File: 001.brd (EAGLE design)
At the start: 100 x 80 mm, 16 parts, among them IC1 74HC148N

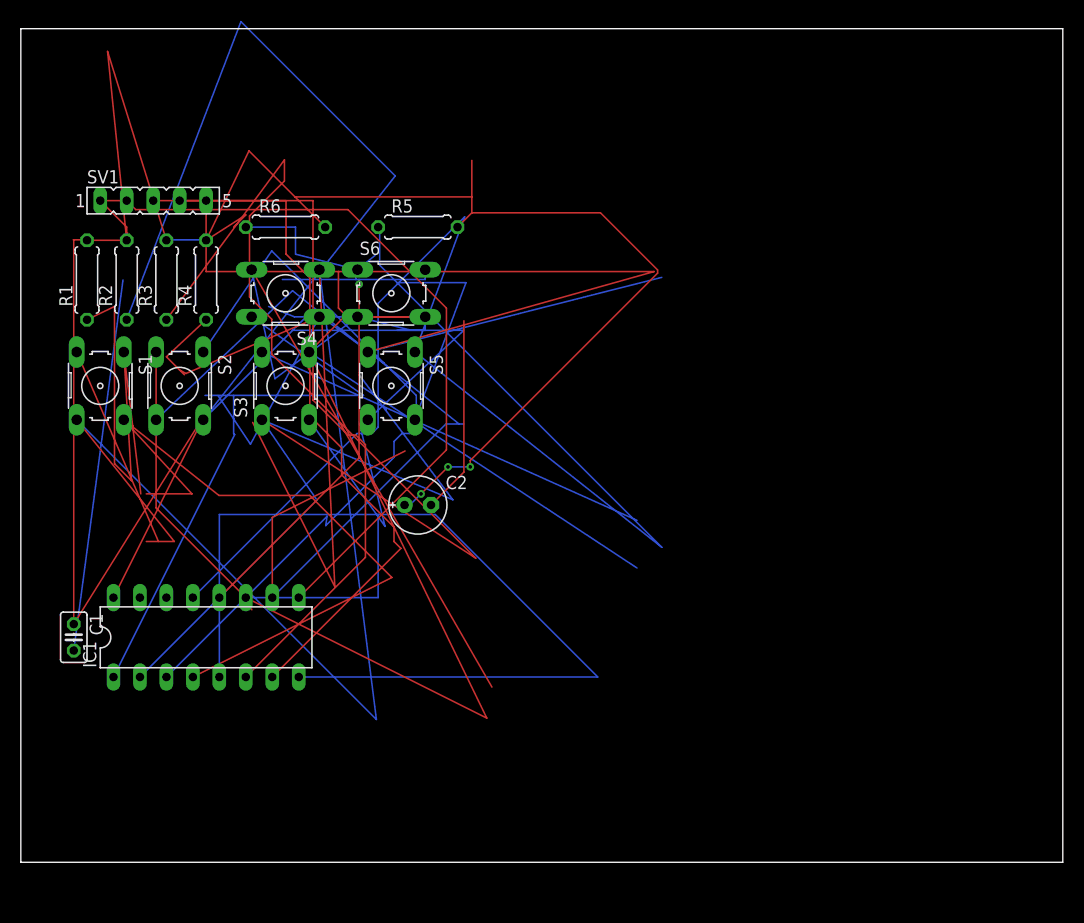
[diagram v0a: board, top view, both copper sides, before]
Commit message: PCB パターンそれなりに完成
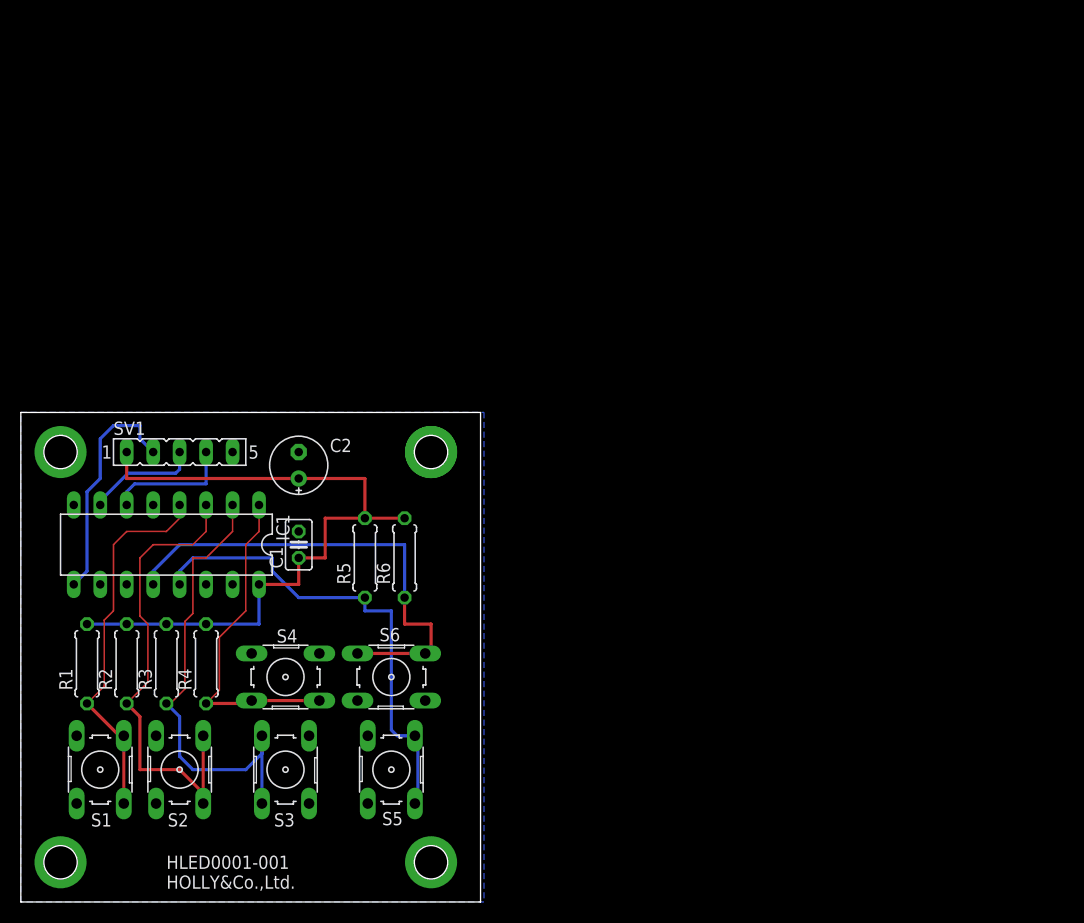
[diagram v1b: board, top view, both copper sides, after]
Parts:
- moved R1 36.8 mm to (6.35, 19.1)
- moved R2 36.8 mm to (10.2, 19.1)
- moved R3 36.8 mm to (14.0, 19.1)
- moved R4 36.8 mm to (17.8, 19.1)
- moved S1 36.8 mm to (7.62, 8.89)
- moved S2 36.8 mm to (15.2, 8.89)
- moved S3 36.8 mm to (25.4, 8.89)
- moved S4 36.8 mm to (25.4, 17.8)
- moved S5 36.8 mm to (35.6, 8.89)
- moved S6 36.8 mm to (35.6, 17.8)
- moved R6 33.7 mm to (36.8, 29.2), turned to 90 degrees
- moved R5 32.2 mm to (33.0, 29.2), turned to 90 degrees
- moved SV1 24.3 mm to (15.2, 39.4)
- moved C1 23.3 mm to (26.7, 30.5), turned to 90 degrees
- moved C2 12.0 mm to (26.7, 38.1), turned to 90 degrees
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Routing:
- net GND: track 818.8 -> 0.00 mm, vias 0 -> 5
- net VCC: track 239.3 -> 69.9 mm, vias 3 -> 0
- net N$4: track 200.0 -> 45.5 mm
- net N$3: track 175.3 -> 46.4 mm
- net N$6: track 155.0 -> 46.4 mm
- net N$2: track 113.4 -> 36.3 mm
- net N$5: track 99.9 -> 32.1 mm
- net N$9: track 68.2 -> 10.9 mm
- net N$10: track 65.8 -> 12.3 mm
- net N$8: track 68.6 -> 22.4 mm
- net N$7: track 67.6 -> 46.2 mm, vias 1 -> 0
- added copper zone on layer 16, net GND
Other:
- board size 100 x 80 mm -> 44.1 x 47 mm
- board text added: "HLED0001-001 HOLLY&Co.,Ltd."
